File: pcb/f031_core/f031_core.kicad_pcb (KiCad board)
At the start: 2 copper layers, 55.9 x 36.8 mm, 31 parts, among them J1 Conn_02x13_Odd_Even, J2 Conn_02x13_Odd_Even, J3 USB_B_Mini, J4 Conn_01x04, J5 Conn_02x03_Odd_Even, SW1 SW_Push, U1 STM32F031C6Tx, U2 AMS1117-3.3, Y1 8M, Y2 32768HZ

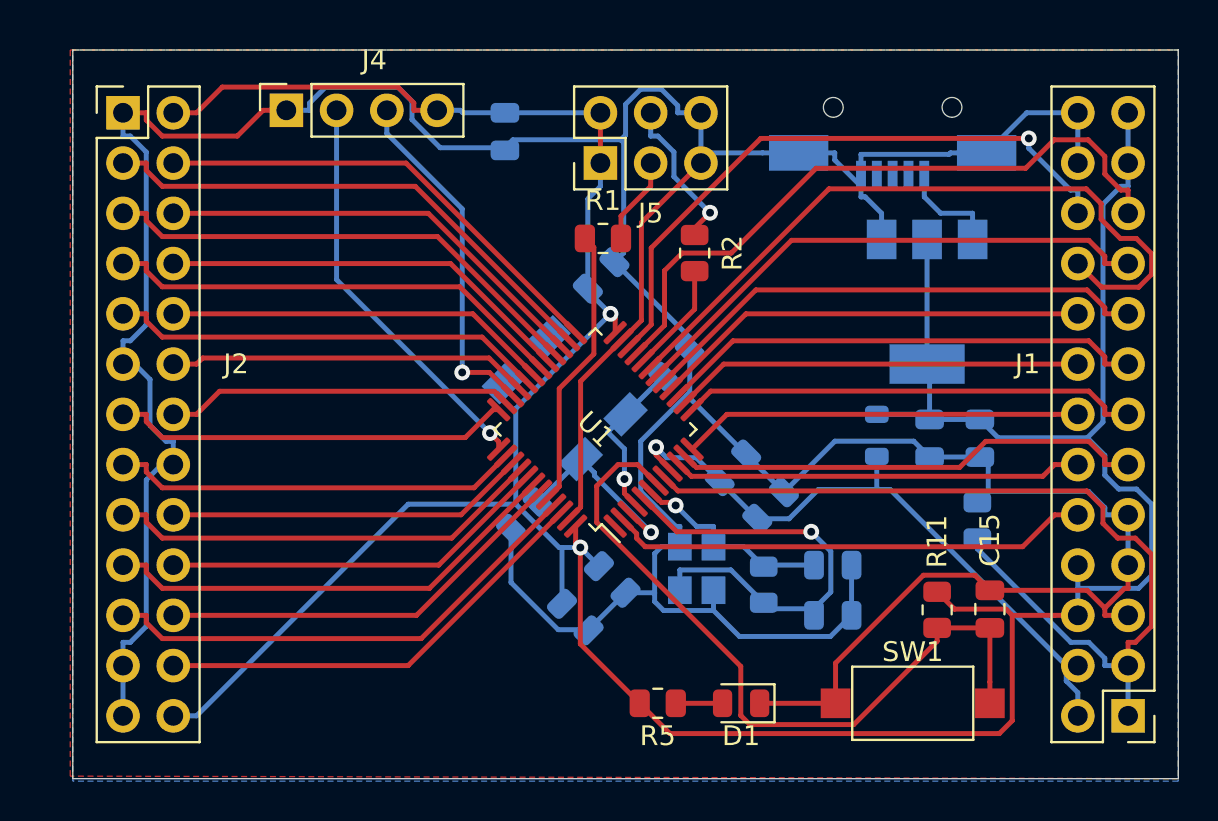
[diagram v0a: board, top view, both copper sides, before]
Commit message: Update f031_core board.
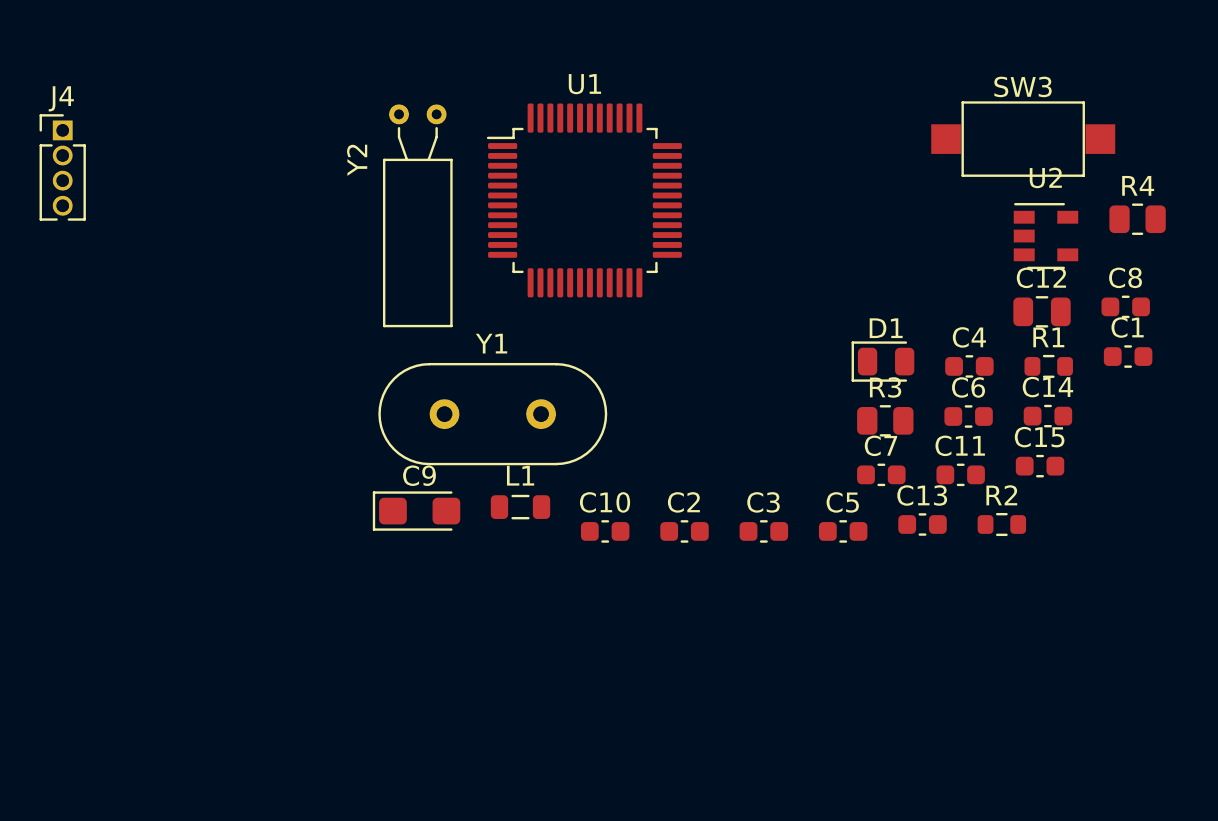
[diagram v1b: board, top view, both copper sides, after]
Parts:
- removed J1, J2: Conn_02x13_Odd_Even, Connector_PinHeader_2.54mm:PinHeader_2x13_P2.54mm_Vertical
- removed J3: USB_B_Mini, Connector_USB:USB_Mini-B_AdamTech_MUSB-B5-S-VT-TSMT-1_SMD_Vertical
- removed J5: Conn_02x03_Odd_Even, Connector_PinHeader_2.54mm:PinHeader_2x03_P2.54mm_Vertical
- removed R11, R5: 510R, Resistor_SMD:R_0805_2012Metric
- removed SW1: SW_Push, Button_Switch_SMD:SW_SPST_CK_RS282G05A3
- added C13: 100nF, Capacitor_SMD:C_0603_1608Metric, F.Cu at (93.8, 62.1)
- added C14: 1uF, Capacitor_SMD:C_0603_1608Metric, F.Cu at (100.1, 56.6)
- added SW3: SW_Push, Button_Switch_SMD:SW_SPST_CK_RS282G05A3, F.Cu at (98.8, 42.6)
- C1, C2: footprint Capacitor_SMD:C_0805_2012Metric -> Capacitor_SMD:C_0603_1608Metric; moved to F.Cu
- C10: value 10nF -> 100nF; footprint Capacitor_SMD:C_0805_2012Metric -> Capacitor_SMD:C_0603_1608Metric; moved to F.Cu
- C11: value 10uF -> 100nF; footprint Capacitor_SMD:C_0805_2012Metric -> Capacitor_SMD:C_0603_1608Metric; moved to F.Cu
- C12: value 0.1uF -> 4.7uF; moved to F.Cu
- C15: value 10pF -> 10nF; footprint Capacitor_SMD:C_0805_2012Metric -> Capacitor_SMD:C_0603_1608Metric
- C3, C4: value 20pF -> 10pF; footprint Capacitor_SMD:C_0805_2012Metric -> Capacitor_SMD:C_0603_1608Metric; moved to F.Cu
- C5: value 0.1uF -> 100nF; footprint Capacitor_SMD:C_0805_2012Metric -> Capacitor_SMD:C_0603_1608Metric; moved to F.Cu
- C6: value 0.1uF -> 10uF; footprint Capacitor_SMD:C_0805_2012Metric -> Capacitor_SMD:C_0603_1608Metric; moved to F.Cu
- C7: value 4.7uF -> 100nF; footprint Capacitor_SMD:C_0805_2012Metric -> Capacitor_SMD:C_0603_1608Metric; moved to F.Cu
- C8: value 0.1uF -> 470pF; footprint Capacitor_SMD:C_0805_2012Metric -> Capacitor_SMD:C_0603_1608Metric; moved to F.Cu
- C9: value 1uF -> 2.2uF; footprint Capacitor_SMD:C_0805_2012Metric -> Capacitor_Tantalum_SMD:CP_EIA-3216-18_Kemet-A; moved to F.Cu
- J4: footprint Connector_PinSocket_2.54mm:PinSocket_1x04_P2.54mm_Vertical -> Connector_PinHeader_1.27mm:PinHeader_1x04_P1.27mm_Vertical
- L1, R4: moved to F.Cu
- R1: value 100K -> 10K; footprint Resistor_SMD:R_0805_2012Metric -> Resistor_SMD:R_0603_1608Metric
- R2: value 100K -> 390; footprint Resistor_SMD:R_0805_2012Metric -> Resistor_SMD:R_0603_1608Metric
- R3: value 10M -> 510R; moved to F.Cu
- U2: value AMS1117-3.3 -> MIC5219-3.3YM5; footprint Package_TO_SOT_SMD:SOT-223-3_TabPin2 -> Package_TO_SOT_SMD:SOT-23-5; moved to F.Cu
- Y1: footprint Crystal:Crystal_SMD_3225-4Pin_3.2x2.5mm -> Crystal:Crystal_HC49-4H_Vertical; moved to F.Cu
- Y2: value 32768HZ -> 32.768; footprint Crystal:Crystal_SMD_Abracon_ABS25-4Pin_8.0x3.8mm -> Crystal:Crystal_C38-LF_D3.0mm_L8.0mm_Horizontal; moved to F.Cu
- moved C8 29.4 mm to (104.0, 51.1), turned to 0 degrees
- moved C5 26.5 mm to (89.7, 62.4), turned to 0 degrees
- moved R1 23.4 mm to (100.1, 54.1), turned to 0 degrees
- moved R2 20.7 mm to (97.8, 62.1), turned to 0 degrees
- moved C6 19.9 mm to (96.1, 56.6), turned to 0 degrees
- moved C1 19.8 mm to (104.1, 53.6), turned to 0 degrees
- moved D1 18.8 mm to (91.9, 53.8), turned to 0 degrees
- moved L1 18.4 mm to (73.4, 61.2), turned to 0 degrees
- moved C9 17.7 mm to (68.3, 61.4), turned to 0 degrees
- moved R4 17.2 mm to (104.6, 46.7), turned to 0 degrees
- moved C7 17.1 mm to (91.7, 59.6), turned to 0 degrees
- moved Y2 16.6 mm to (67.3, 41.4), turned to 0 degrees
- moved Y1 14.9 mm to (69.6, 56.5), turned to 0 degrees
- moved C4 14.8 mm to (96.1, 54.1), turned to 0 degrees
- moved C3 12.1 mm to (85.7, 62.4), turned to 0 degrees
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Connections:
- net Net-(U1-Pad1) renamed VBAT
- C10 pad 1: +3.3VA -> RESET
- C15 pad 1: RESET -> +3.3VA
- C6 pad 1: +3V3 -> VCC
- C7 pad 1: +3V3 -> VCC
- C8 pad 1: +3V3 -> Net-(C8-Pad1)
- C9 pad 1: +3.3VA -> +3V3
- L1 pad 1: +3V3 -> +3.3VA
- L1 pad 2: +3.3VA -> +3V3
- R2 pad 1: /BOOT1 -> /RCC_OSC_OUT
- R2 pad 2: Net-(J5-Pad4) -> /RCC_OSC_IN
- R3 pad 1: /RCC_OSC_OUT -> Net-(D1-Pad2)
- R3 pad 2: /RCC_OSC_IN -> +3V3
- U2 pad 1: GND -> VCC
- U2 pad 2: +3V3 -> GND
- Y1 pad 2: GND -> /RCC_OSC_OUT
- Y2 pad 2: Net-(Y2-Pad2) -> /RCC_OSC32_OUT
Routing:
- net GND: track 235.3 -> 0.00 mm
- net +3V3: track 173.0 -> 0.00 mm, vias 2 -> 0
- net GNDA: track 46.4 -> 0.00 mm
- net RESET: track 37.5 -> 0.00 mm
- net /PB1: track 36.4 -> 0.00 mm
- net /PB10: track 33.7 -> 0.00 mm
- net +3.3VA: track 33.0 -> 0.00 mm, vias 1 -> 0
- net /PB11: track 31.9 -> 0.00 mm, vias 1 -> 0
- net /PB0: track 27.3 -> 0.00 mm
- net /PB13: track 26.4 -> 0.00 mm
- net /PA7: track 26.1 -> 0.00 mm
- net /PB8: track 25.3 -> 0.00 mm
- net /PB15: track 25.0 -> 0.00 mm
- net /PA5: track 24.6 -> 0.00 mm
- net /PC13: track 24.4 -> 0.00 mm
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- removed copper zone on B.Cu, net GND
- removed copper zone on F.Cu, net GND
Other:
- board outline removed
